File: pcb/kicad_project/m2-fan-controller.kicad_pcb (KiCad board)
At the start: 2 copper layers, 22 x 30 mm, 17 parts, among them J1 Bus_M.2_Socket_E, J2 Conn_01x04, J3 Conn_01x04, J4 JST PH_S2B-PH-K, U1 STM32F042F6P6

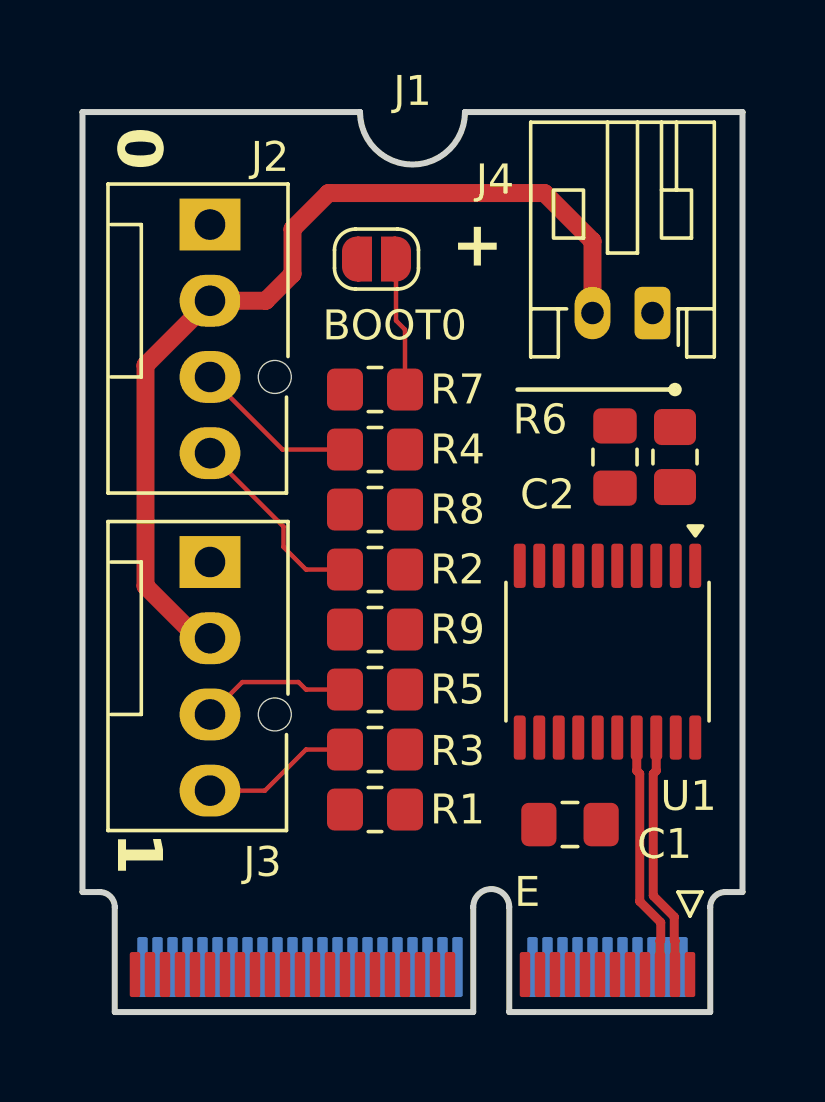
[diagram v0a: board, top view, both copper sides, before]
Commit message: Hopefully final revision
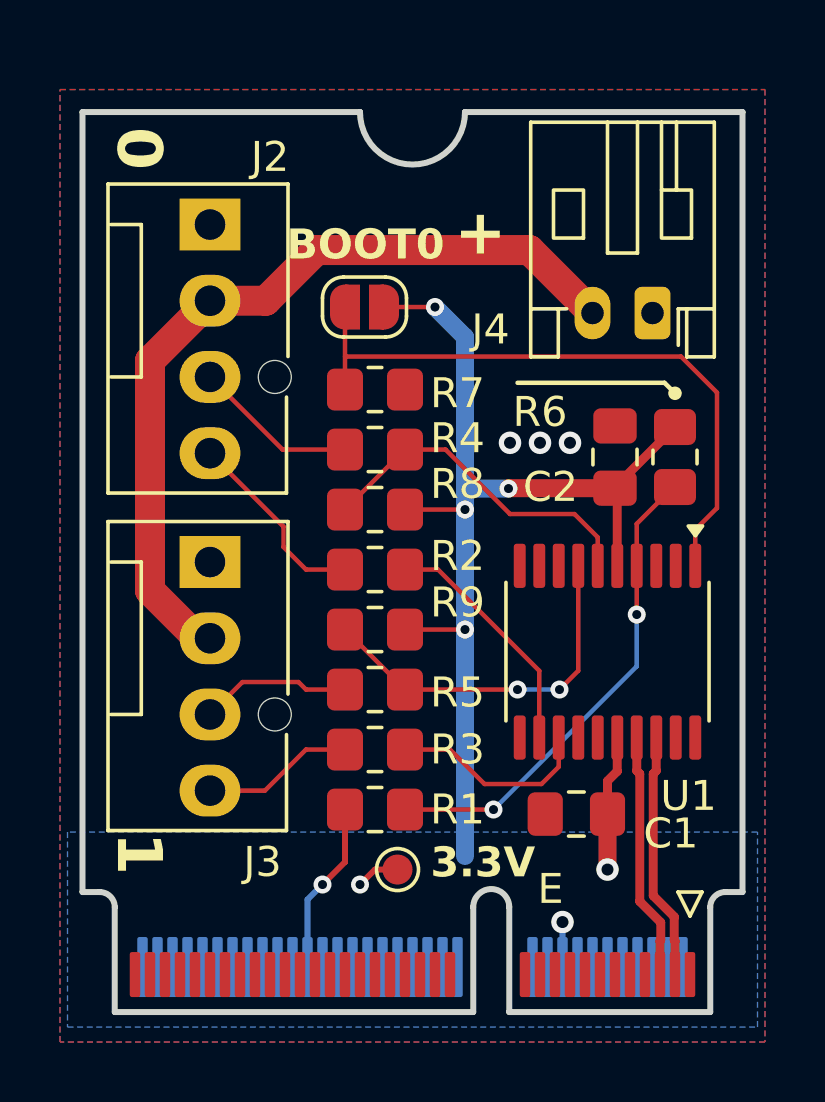
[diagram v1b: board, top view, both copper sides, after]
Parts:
- added TP1: TestPoint, TestPoint:TestPoint_Pad_D1.0mm, F.Cu at (138.5, 105.2)
- moved JP1 1.65 mm to (137.4, 86.5), turned to 180 degrees
- moved C1 0.41 mm to (144.5, 103.4)
- turned R7 to 0 degrees
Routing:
- net +3.3V: track 0.00 -> 40.5 mm, vias 0 -> 6
- net BOOT0: track 4.47 -> 21.7 mm
- net RST: track 0.00 -> 16.2 mm, vias 0 -> 2
- net TACH_1: track 0.00 -> 12.9 mm, vias 0 -> 2
- net TACH_0: track 0.00 -> 11.4 mm
- net PWM_0: track 0.00 -> 8.10 mm
- net PWM_1: track 0.00 -> 6.81 mm
- net Net-(J1-~{PERST0}): track 0.00 -> 5.77 mm, vias 0 -> 1
- net +12V: track 31.4 -> 27.5 mm
- net GND: track 0.00 -> 1.50 mm, vias 0 -> 4
- added copper zone on B.Cu, net +3.3V
- added copper zone on B.Cu, net GND
- added copper zone on F.Cu, net GND
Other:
- board text added: "(c) 2026 - Sergio Carmine"
- board text added: "3.3V"
- board text added: "M.2 fan controller"
